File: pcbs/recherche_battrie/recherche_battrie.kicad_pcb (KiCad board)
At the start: 2 copper layers, 24 x 9 mm, 12 parts, among them J1 Conn_01x02, J2 Conn_01x02, Q1 PMOS, SW1 SW_Push, U1 LP5907MFX-3.3, U4 TPL5110

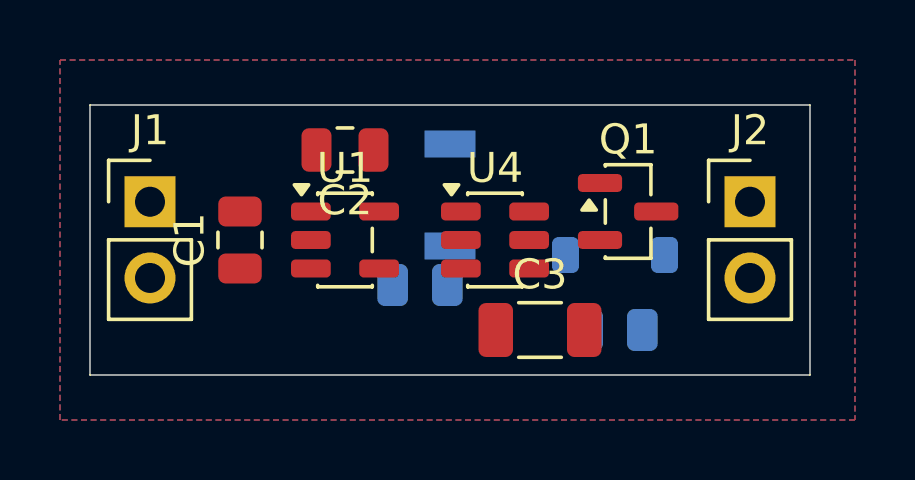
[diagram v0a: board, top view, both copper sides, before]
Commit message: pcb rcharge battrie
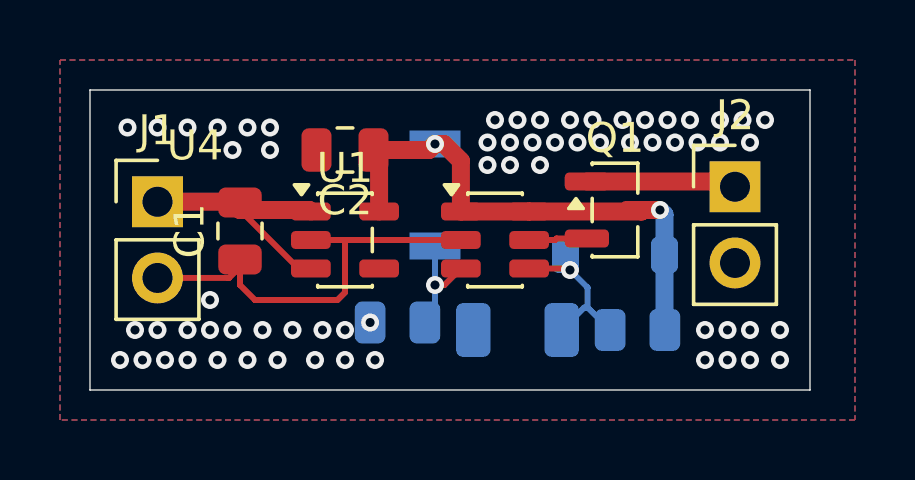
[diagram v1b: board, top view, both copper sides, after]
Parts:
- C3: moved to B.Cu
- moved R1 1.46 mm to (46.8, 55.8)
- moved C3 0.75 mm to (50.8, 56.0)
- moved R2 0.75 mm to (54.8, 56.0)
- moved J2 0.71 mm to (58.0, 51.2)
- moved SW1 0.50 mm to (48.0, 51.5)
- moved Q1 0.44 mm to (54.0, 52.0)
- moved C1 0.30 mm to (41.5, 52.7)
- moved J1 0.25 mm to (38.8, 51.7)
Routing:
- net +3V3: track 0.00 -> 16.5 mm, vias 0 -> 2
- net GND: track 0.00 -> 14.6 mm, vias 0 -> 64
- net /bat+: track 0.00 -> 8.67 mm
- net Net-(J2-Pin_1): track 0.00 -> 5.72 mm
- net Net-(D1-A): track 0.00 -> 5.11 mm, vias 0 -> 1
- net Net-(U4-DELAY/M_DRV): track 0.00 -> 3.93 mm, vias 0 -> 1
- net Net-(Q1-G): track 0.00 -> 1.95 mm
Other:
- board size 24 x 9 mm -> 24 x 10 mm
